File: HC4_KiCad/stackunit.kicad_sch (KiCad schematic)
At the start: 18 parts, among them IC11 74HC161, IC12 74HC377

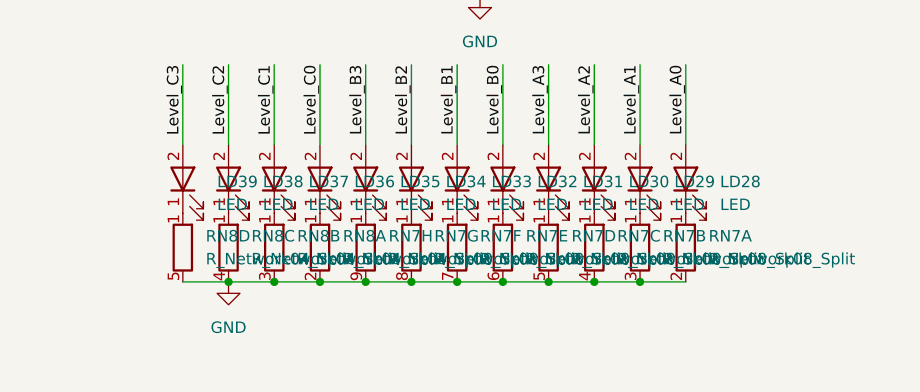
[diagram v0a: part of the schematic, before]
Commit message: 電源配線ほぼ完了
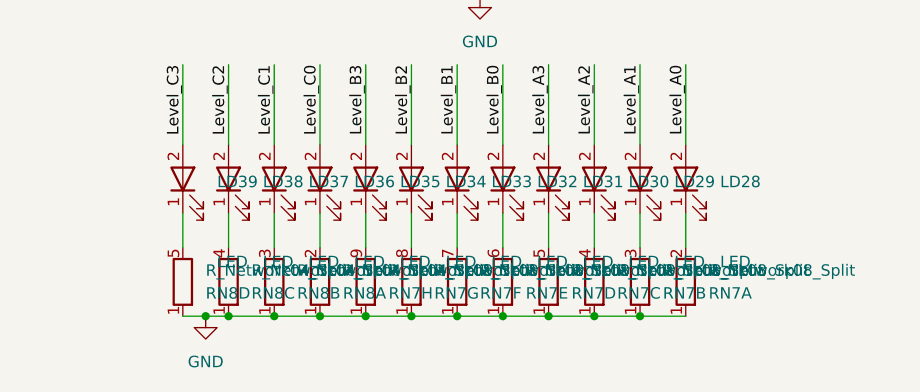
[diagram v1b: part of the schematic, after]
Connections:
- net GND: now also RN7.1 (R1), RN7.1 (R1), RN7.1 (R1), RN7.1 (R1), RN7.1 (R1), RN7.1 (R1), RN7.1 (R1), RN7.1 (R1), RN8.1 (R1), RN8.1 (R1), RN8.1 (R1), RN8.1 (R1); no longer RN7.2 (R1.2), RN7.3 (R2.2), RN7.4 (R3.2), RN7.5 (R4.2), RN7.6 (R5.2), RN7.7 (R6.2), RN7.8 (R7.2), RN7.9 (R8.2), RN8.2 (R1.2), RN8.3 (R2.2), RN8.4 (R3.2), RN8.5 (R4.2)
- net at LD37.1 (K): now also RN8.3 (R2.2); no longer RN8.1 (R1)
- net at LD36.1 (K): now also RN8.2 (R1.2); no longer RN8.1 (R1)
- net at LD28.1 (K): now also RN7.2 (R1.2); no longer RN7.1 (R1)
- net at LD29.1 (K): now also RN7.3 (R2.2); no longer RN7.1 (R1)
- net at LD35.1 (K): now also RN7.9 (R8.2); no longer RN7.1 (R1)
- net at LD30.1 (K): now also RN7.4 (R3.2); no longer RN7.1 (R1)
- net at LD32.1 (K): now also RN7.6 (R5.2); no longer RN7.1 (R1)
- net at LD39.1 (K): now also RN8.5 (R4.2); no longer RN8.1 (R1)
- net at LD31.1 (K): now also RN7.5 (R4.2); no longer RN7.1 (R1)
- net at LD33.1 (K): now also RN7.7 (R6.2); no longer RN7.1 (R1)
- net at LD34.1 (K): now also RN7.8 (R7.2); no longer RN7.1 (R1)
- net at LD38.1 (K): now also RN8.4 (R3.2); no longer RN8.1 (R1)
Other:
- moved on the sheet: RN7A, RN7B, RN7C, RN7D, RN7E, RN7F, RN7G, RN7H, RN8A, RN8B, RN8C, RN8D
